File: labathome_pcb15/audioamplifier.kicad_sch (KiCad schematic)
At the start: 33 parts, among them U1 TAS5805M

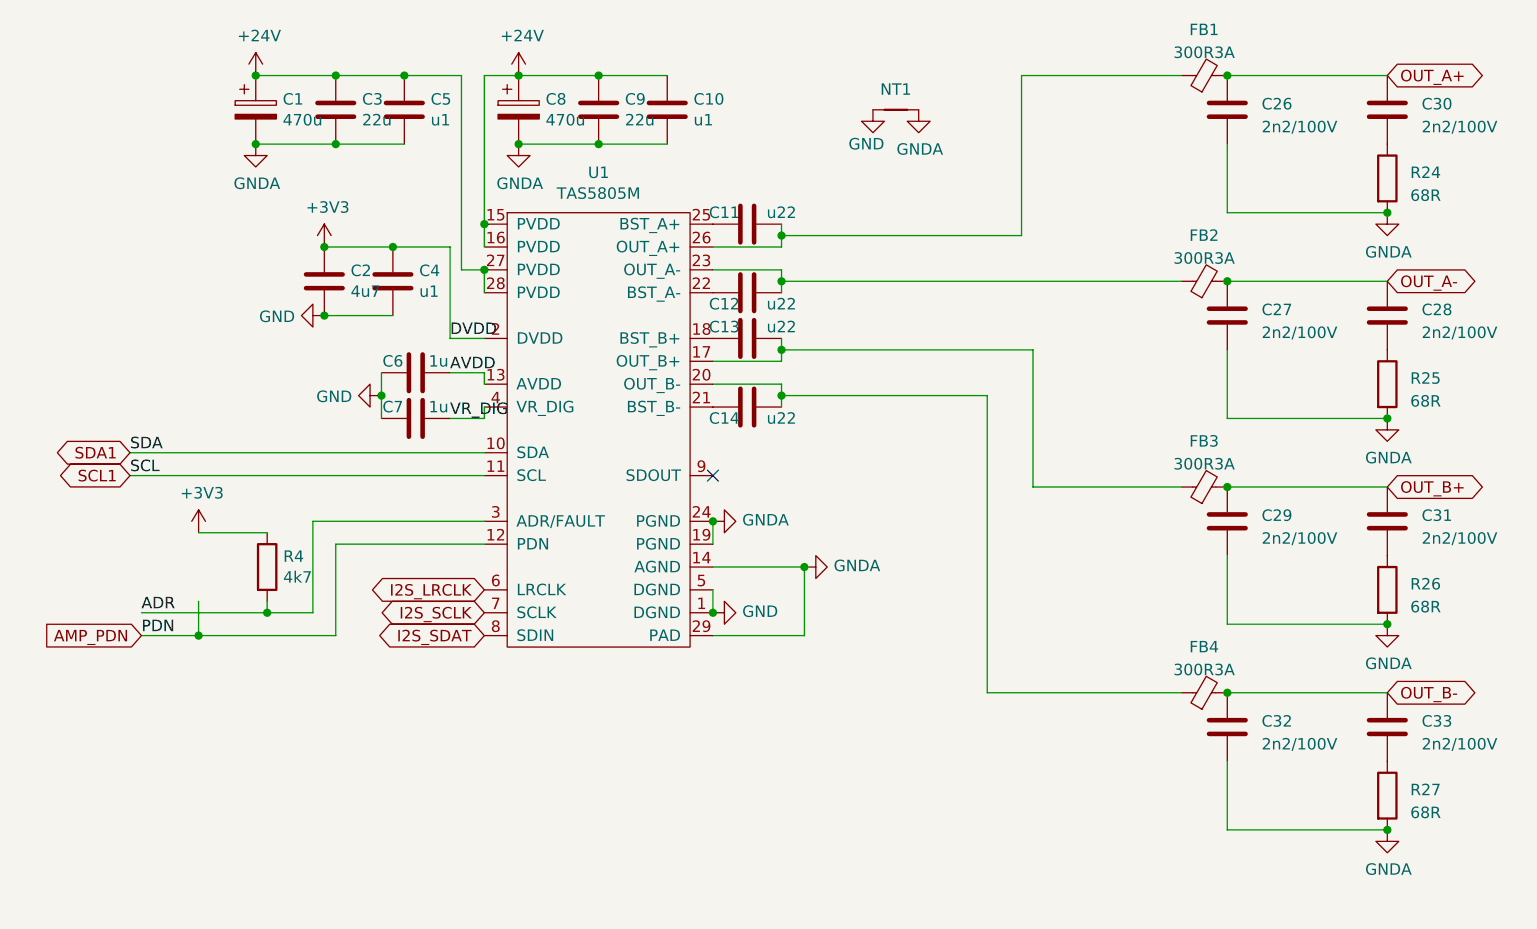
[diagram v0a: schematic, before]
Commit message: PCB_v15 wip
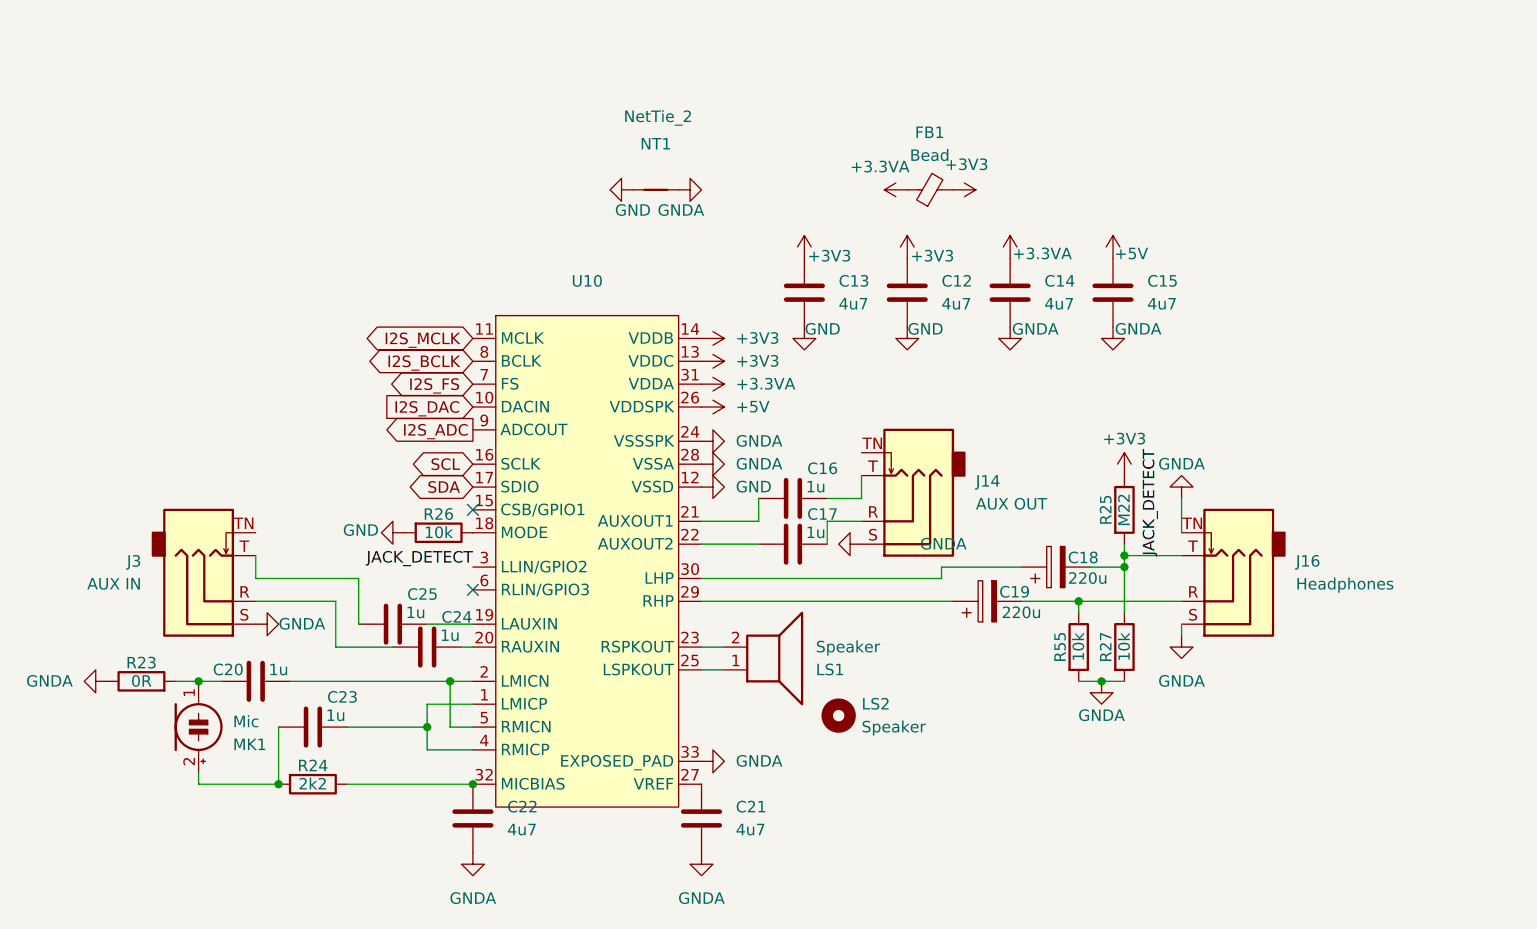
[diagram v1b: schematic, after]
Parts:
- removed C1, C8: 470u, Capacitor_THT:CP_Radial_D10.0mm_P3.50mm, symbol Device:CP
- removed C10, C5: u1, Capacitor_SMD:C_0603_1608Metric, symbol Device:C
- removed C11: u22, Capacitor_SMD:C_0603_1608Metric, symbol Device:C
- removed C2: 4u7, Capacitor_SMD:C_0402_1005Metric, symbol Device:C
- removed C26, C27, C28, C29, C30, C31, C32, C33: 2n2/100V, Capacitor_SMD:C_0603_1608Metric, symbol Device:C
- removed C3, C9: 22u, Capacitor_SMD:C_1210_3225Metric_Pad1.33x2.70mm_HandSolder, symbol Device:C
- removed C4: u1, Capacitor_SMD:C_0402_1005Metric, symbol Device:C
- removed C6, C7: 1u, Capacitor_SMD:C_0402_1005Metric, symbol Device:C
- removed FB2, FB3, FB4: 300R3A, Resistor_SMD:R_1206_3216Metric, symbol Device:FerriteBead_Small
- removed NT1: Net-Tie_2, NetTie:NetTie-2_SMD_Pad2.0mm, symbol Device:Net-Tie_2
- removed R4: 4k7, Resistor_SMD:R_0402_1005Metric, symbol Device:R
- removed U1: TAS5805M, Package_SO:HTSSOP-28-1EP_4.4x9.7mm_P0.65mm_EP2.85x5.4mm_ThermalVias, symbol liebler_SEMICONDUCTORS:TAS5805M
- added C15, C21, C22: 4u7, Capacitor_SMD:C_0402_1005Metric, symbol Device:C
- added C16, C17, C20, C23, C24, C25: 1u, Capacitor_SMD:C_0402_1005Metric, symbol Device:C
- added C18, C19: 220u, Capacitor_SMD:CP_Elec_6.3x5.4, symbol Device:C_Polarized
- added J14: AUX OUT, liebler_CONN:PJ-327A, symbol Connector_Audio:AudioJack3_SwitchT
- added J16: Headphones, liebler_CONN:PJ-327A, symbol Connector_Audio:AudioJack3_SwitchT
- added J3: AUX IN, liebler_CONN:PJ-327A, symbol Connector_Audio:AudioJack3_SwitchT
- added LS1: Speaker, Connector_PinHeader_2.00mm:PinHeader_1x02_P2.00mm_Vertical, symbol Device:Speaker
- added LS2: Speaker, liebler_MECH:SPEAKER_2415, symbol Mechanical:MountingHole
- added MK1: Mic, liebler_PASSIVES:Microphone_6mm, symbol Device:Microphone_Condenser
- added NT1: NetTie_2, NetTie:NetTie-2_SMD_Pad0.5mm, symbol Device:NetTie_2
- added R23: 0R, Resistor_SMD:R_0402_1005Metric, symbol Device:R
- added R55: 10k, Resistor_SMD:R_0402_1005Metric, symbol Device:R
- added U10: ~, Package_DFN_QFN:QFN-32-1EP_5x5mm_P0.5mm_EP3.6x3.6mm_ThermalVias, symbol liebler_SEMICONDUCTORS:NAU88C22
- C12, C13, C14: value u22 -> 4u7; footprint Capacitor_SMD:C_0603_1608Metric -> Capacitor_SMD:C_0402_1005Metric
- FB1: value 300R3A -> Bead; footprint Resistor_SMD:R_1206_3216Metric -> Inductor_SMD:L_0603_1608Metric
- R24: value 68R -> 2k2; footprint Resistor_SMD:R_0603_1608Metric -> Resistor_SMD:R_0402_1005Metric
- R25: value 68R -> M22; footprint Resistor_SMD:R_0603_1608Metric -> Resistor_SMD:R_0402_1005Metric
- R26, R27: value 68R -> 10k; footprint Resistor_SMD:R_0603_1608Metric -> Resistor_SMD:R_0402_1005Metric
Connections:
- net OUT_A+ is gone; now on net +3V3: FB1.2
- net +3V3: now also C12.1, C13.1, R25.1, U10.13 (VDDC), U10.14 (VDDB)
- net GND: now also C12.2, C13.2, R26.2, NT1.1, U10.12 (VSSD)
- net GNDA: now also C14.2, C15.2, C21.2, C22.2, J14.S, J16.S, J16.TN, J3.S, NT1.2, R23.1, R55.2, U10.24 (VSSSPK), U10.28 (VSSA), U10.33 (EXPOSED_PAD); no longer R24.2, R25.2, R26.2
- net JACK_DETECT: now reaches R27.1
- net JACK_DETECT: now also R25.2, C18.2, J16.T, U10.3 (LLIN/GPIO2)
- net +3.3VA: now reaches C14.1
- net +3.3VA: now also FB1.1, U10.31 (VDDA)
- net at R24.1: now also C22.1, U10.32 (MICBIAS)
- net at R26.1: now also U10.18 (MODE)
- new net: C17.2, J14.R
- new net: C16.2, J14.T
- new net: C19.1, U10.29 (RHP)
- new net: C19.2, J16.R, R55.1
- new net: C24.1, J3.R
- new net: C24.2, U10.20 (RAUXIN)
- new net: LS1.1, U10.25 (LSPKOUT)
- new net: LS1.2, U10.23 (RSPKOUT)
- new net: C23.1, MK1.2 (+), R24.2
- new net: C25.1, J3.T
- new net: C25.2, U10.19 (LAUXIN)
- new net: C17.1, U10.22 (AUXOUT2)
- new net: C20.1, MK1.1 (-), R23.2
- new net: C18.1, U10.30 (LHP)
- new net: C20.2, U10.2 (LMICN), U10.5 (RMICN)
- new net: C23.2, U10.1 (LMICP), U10.4 (RMICP)
- new net: C21.1, U10.27 (VREF)
- new net: C16.1, U10.21 (AUXOUT1)
- new net +5V: C15.1, U10.26 (VDDSPK)
- new net I2S_ADC: U10.9 (ADCOUT)
- new net I2S_BCLK: U10.8 (BCLK)
- new net I2S_DAC: U10.10 (DACIN)
- new net I2S_FS: U10.7 (FS)
- new net I2S_MCLK: U10.11 (MCLK)
- new net SCL: U10.16 (SCLK)
- new net SDA: U10.17 (SDIO)
- no-connect marks 1 -> 2

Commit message: labathome wip
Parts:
- FB1: footprint Inductor_SMD:L_0603_1608Metric -> Inductor_SMD:L_0603_1608Metric
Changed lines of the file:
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@@
 			)
 		)
-		(property "Footprint" "Inductor_SMD:L_0603_1608Metric "
+		(property "Footprint" "Inductor_SMD:L_0603_1608Metric"
 			(at 125.73 38.608 90)
 			(effects
